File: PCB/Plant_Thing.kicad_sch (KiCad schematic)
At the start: 34 parts, among them J7 VDDH, J8 EXT 3.3V, U1 nRF52820-QDxx, X1 HY32768KSMD3068YA2R30, Y1 32M

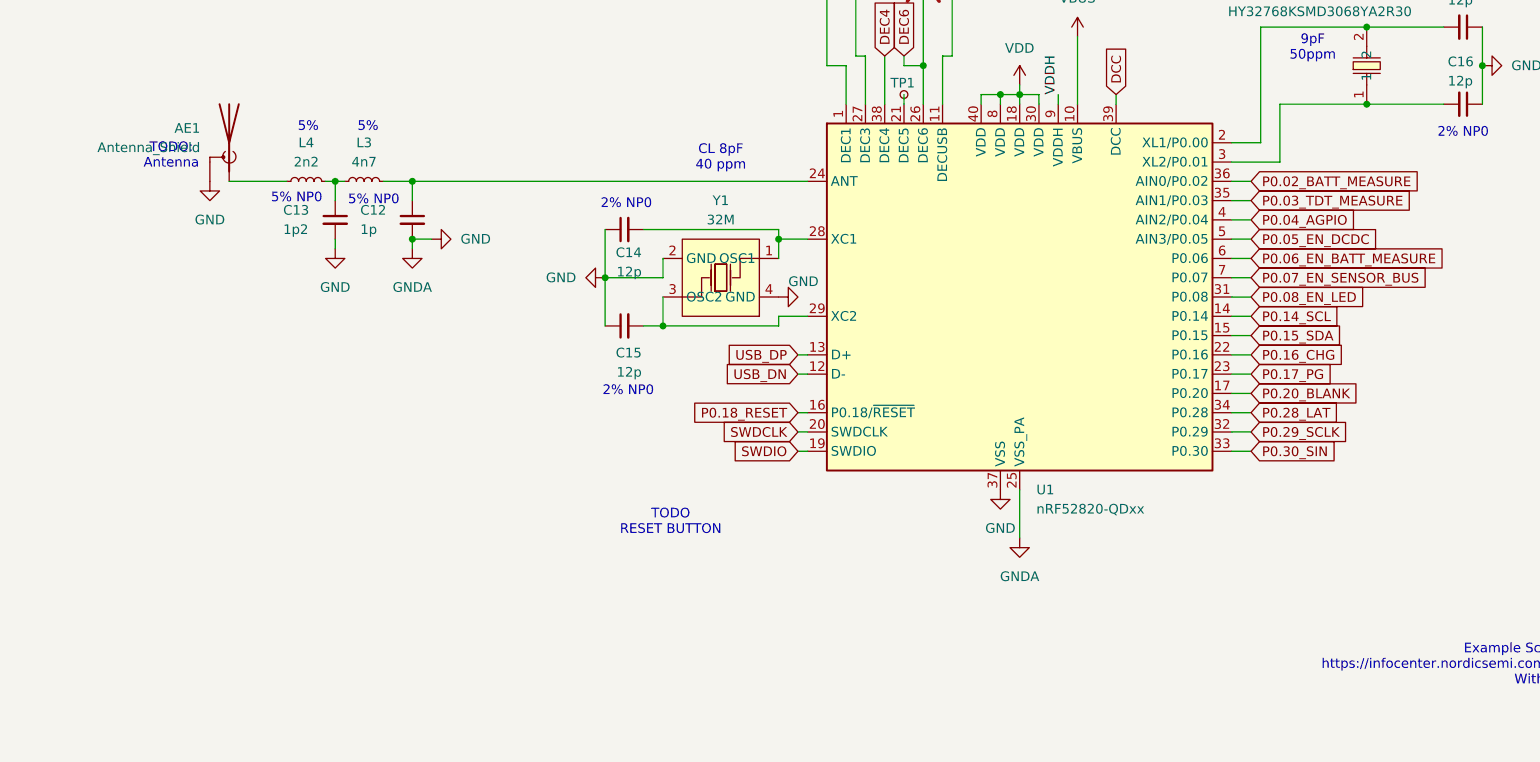
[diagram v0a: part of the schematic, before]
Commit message: Finished Devboard
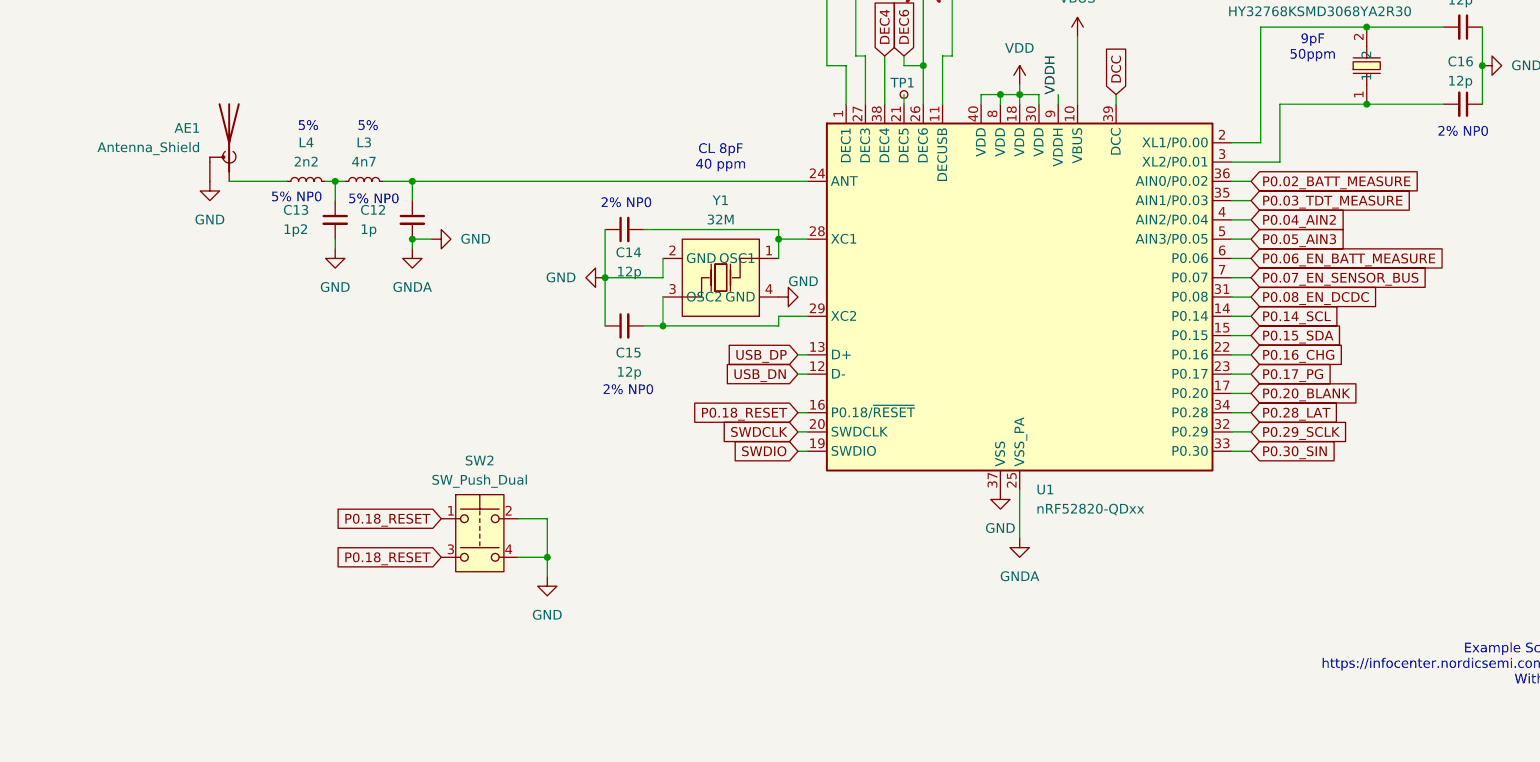
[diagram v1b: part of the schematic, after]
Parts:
- added SW2: SW_Push_Dual, Button_Switch_SMD:SW_Push_1P1T_XKB_TS-1187A, symbol Switch:SW_Push_Dual
- C3: footprint (none) -> Capacitor_SMD:C_0402_1005Metric
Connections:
- net GND: now also SW2.2, SW2.4
- net P0.18_RESET: now also SW2.1, SW2.3
- net P0.04_AGPIO renamed P0.04_AIN2
- net P0.05_EN_DCDC renamed P0.05_AIN3
- net P0.08_EN_LED renamed P0.08_EN_DCDC
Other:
- note removed: "TODO RESET BUTTON"
- note removed: "TODO: Antenna"
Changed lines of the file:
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@@
 	)
 	(junction
+		(at 87.63 146.05)
+		(diameter 0)
+		(color 0 0 0 0)
+	)
+	(junction
 		(at 59.69 96.52)
 		(diameter 0)
@@
 	(wire
 		(pts
+			(xy 87.63 146.05) (xy 87.63 148.59)
+		)
+		(stroke
+			(width 0)
+			(type default)
+		)
+	)
+	(wire
+		(pts
 			(xy 102.87 109.22) (xy 95.25 109.22)
 		)
@@
 	(wire
 		(pts
+			(xy 87.63 140.97) (xy 83.82 140.97)
+		)
+		(stroke
+			(width 0)
+			(type default)
+		)
+	)
+	(wire
+		(pts
 			(xy 177.8 124.46) (xy 180.34 124.46)
 		)
@@
 	(wire
 		(pts
+			(xy 87.63 146.05) (xy 87.63 140.97)
+		)
+		(stroke
+			(width 0)
+			(type default)
+		)
+	)
+	(wire
+		(pts
 			(xy 118.11 115.57) (xy 118.11 114.3)
 		)
@@
 	(wire
 		(pts
+			(xy 177.8 104.14) (xy 180.34 104.14)
+		)
+		(stroke
+			(width 0)
+			(type default)
+		)
+	)
+	(wire
+		(pts
 			(xy 177.8 34.29) (xy 173.99 34.29)
 		)
@@
 	(wire
 		(pts
+			(xy 83.82 146.05) (xy 87.63 146.05)
+		)
+		(stroke
+			(width 0)
+			(type default)
+		)
+	)
+	(wire
+		(pts
 			(xy 124.46 81.28) (xy 124.46 72.39)
 		)
@@
 	(wire
 		(pts
-			(xy 177.8 104.14) (xy 180.34 104.14)
-		)
-		(stroke
-			(width 0)
-			(type default)
-		)
-	)
-	(wire
-		(pts
 			(xy 137.16 81.28) (xy 137.16 86.36)
 		)
@@
 		)
 	)
-	(text "TODO:\nAntenna"
-		(exclude_from_sim no)
-		(at 38.1 93.218 0)
-		(effects
-			(font
-				(size 1.27 1.27)
-			)
-		)
-	)
 	(text "10%\nX7R"
 		(exclude_from_sim no)
@@
 		)
 	)
-	(text "TODO\nRESET BUTTON"
-		(exclude_from_sim no)
-		(at 103.886 141.478 0)
-		(effects
-			(font
-				(size 1.27 1.27)
-			)
-		)
-	)
 	(text "5% NP0"
 		(exclude_from_sim no)
@@
 		)
 	)
-	(global_label "P0.08_EN_LED"
-		(shape input)
-		(at 180.34 111.76 0)
-		(fields_autoplaced yes)
-		(effects
-			(font
-				(size 1.27 1.27)
-			)
-			(justify left)
-		)
-		(property "Intersheetrefs" "${INTERSHEET_REFS}"
-			(at 196.6903 111.76 0)
-			(effects
-				(font
-					(size 1.27 1.27)
-				)
-				(justify left)
-				(hide yes)
-			)
-		)
-	)
 	(global_label "DEC6"
 		(shape input)
@@
 		)
 	)
-	(global_label "P0.04_AGPIO"
+	(global_label "P0.04_AIN2"
 		(shape input)
 		(at 180.34 101.6 0)
@@
 		)
 		(property "Intersheetrefs" "${INTERSHEET_REFS}"
-			(at 195.36 101.6 0)
+			(at 194.0295 101.6 0)
 			(effects
 				(font
@@
 		)
 	)
+	(global_label "P0.18_RESET"
+		(shape input)
+		(at 73.66 146.05 180)
+		(fields_autoplaced yes)
+		(effects
+			(font
+				(size 1.27 1.27)
+			)
+			(justify right)
+		)
+		(property "Intersheetrefs" "${INTERSHEET_REFS}"
+			(at 58.4588 146.05 0)
+			(effects
+				(font
+					(size 1.27 1.27)
+				)
+				(justify right)
+				(hide yes)
+			)
+		)
+	)
 	(global_label "SWDCLK"
 		(shape input)
@@
 		)
 	)
-	(global_label "P0.05_EN_DCDC"
+	(global_label "P0.08_EN_DCDC"
 		(shape input)
-		(at 180.34 104.14 0)
+		(at 180.34 111.76 0)
 		(fields_autoplaced yes)
 		(effects
@@
 		)
 		(property "Intersheetrefs" "${INTERSHEET_REFS}"
-			(at 198.3232 104.14 0)
+			(at 198.3232 111.76 0)
 			(effects
 				(font
@@
 		)
 	)
+	(global_label "P0.05_AIN3"
+		(shape input)
+		(at 180.34 104.14 0)
+		(fields_autoplaced yes)
+		(effects
+			(font
+				(size 1.27 1.27)
+			)
+			(justify left)
+		)
+		(property "Intersheetrefs" "${INTERSHEET_REFS}"
+			(at 194.0295 104.14 0)
+			(effects
+				(font
+					(size 1.27 1.27)
+				)
+				(justify left)
+				(hide yes)
+			)
+		)
+	)
+	(global_label "P0.18_RESET"
+		(shape input)
+		(at 73.66 140.97 180)
+		(fields_autoplaced yes)
+		(effects
+			(font
+				(size 1.27 1.27)
+			)
+			(justify right)
+		)
+		(property "Intersheetrefs" "${INTERSHEET_REFS}"
+			(at 58.4588 140.97 0)
+			(effects
+				(font
+					(size 1.27 1.27)
+				)
+				(justify right)
+				(hide yes)
+			)
+		)
+	)
 	(global_label "DEC6"
 		(shape input)
@@
 	)
 	(symbol
+		(lib_id "power:GND")
+		(at 87.63 148.59 0)
+		(unit 1)
+		(exclude_from_sim no)
+		(in_bom yes)
+		(on_board yes)
+		(dnp no)
+		(fields_autoplaced yes)
+		(property "Reference" "#PWR067"
+			(at 87.63 154.94 0)
+			(effects
+				(font
+					(size 1.27 1.27)
+				)
+				(hide yes)
+			)
+		)
+		(property "Value" "GND"
+			(at 87.63 153.67 0)
+			(effects
+				(font
+					(size 1.27 1.27)
+				)
+			)
+		)
+		(property "Footprint" ""
+			(at 87.63 148.59 0)
+			(effects
+				(font
+					(size 1.27 1.27)
+				)
+				(hide yes)
+			)
+		)
+		(property "Datasheet" ""
+			(at 87.63 148.59 0)
+			(effects
+				(font
+					(size 1.27 1.27)
+				)
+				(hide yes)
+			)
+		)
+		(property "Description" "Power symbol creates a global label with name \"GND\" , ground"
+			(at 87.63 148.59 0)
+			(effects
+				(font
+					(size 1.27 1.27)
+				)
+				(hide yes)
+			)
+		)
+		(pin "1"
+		)
+		(instances
+			(project "Plant_Thing"
+				(path "/3604ffe7-6852-4862-a71a-75c04c0147cb"
+					(reference "#PWR067")
+					(unit 1)
+				)
+			)
+		)
+	)
+	(symbol
 		(lib_id "Mechanical:MountingHole")
 		(at 160.02 195.58 0)
@@
 	)
 	(symbol
+		(lib_id "Switch:SW_Push_Dual")
+		(at 78.74 143.51 0)
+		(unit 1)
+		(exclude_from_sim no)
+		(in_bom yes)
+		(on_board yes)
+		(dnp no)
+		(fields_autoplaced yes)
+		(property "Reference" "SW2"
+			(at 78.74 133.35 0)
+			(effects
+				(font
+					(size 1.27 1.27)
+				)
+			)
+		)
+		(property "Value" "SW_Push_Dual"
+			(at 78.74 135.89 0)
+			(effects
+				(font
+					(size 1.27 1.27)
+				)
+			)
+		)
+		(property "Footprint" "Button_Switch_SMD:SW_Push_1P1T_XKB_TS-1187A"
+			(at 78.74 135.89 0)
+			(effects
+				(font
+					(size 1.27 1.27)
+				)
+				(hide yes)
+			)
+		)
+		(property "Datasheet" "~"
+			(at 78.74 143.51 0)
+			(effects
+				(font
+					(size 1.27 1.27)
+				)
+				(hide yes)
+			)
+		)
+		(property "Description" "Push button switch, generic, symbol, four pins"
+			(at 78.74 143.51 0)
+			(effects
+				(font
+					(size 1.27 1.27)
+				)
+				(hide yes)
+			)
+		)
+		(pin "2"
+		)
+		(pin "1"
+		)
+		(pin "4"
+		)
+		(pin "3"
+		)
+		(instances
+			(project "Plant_Thing"
+				(path "/3604ffe7-6852-4862-a71a-75c04c0147cb"
+					(reference "SW2")
+					(unit 1)
+				)
+			)
+		)
+	)
+	(symbol
 		(lib_id "Device:C_Small")
 		(at 137.16 69.85 0)
@@
 			)
 		)
-		(property "Footprint" ""
+		(property "Footprint" "Capacitor_SMD:C_0402_1005Metric"
 			(at 137.16 69.85 0)
 			(effects
